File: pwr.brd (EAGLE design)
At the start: 50 x 58 mm, 40 parts, among them Q1 IPD65R600E6, T1 750811647, U1 UCC28700

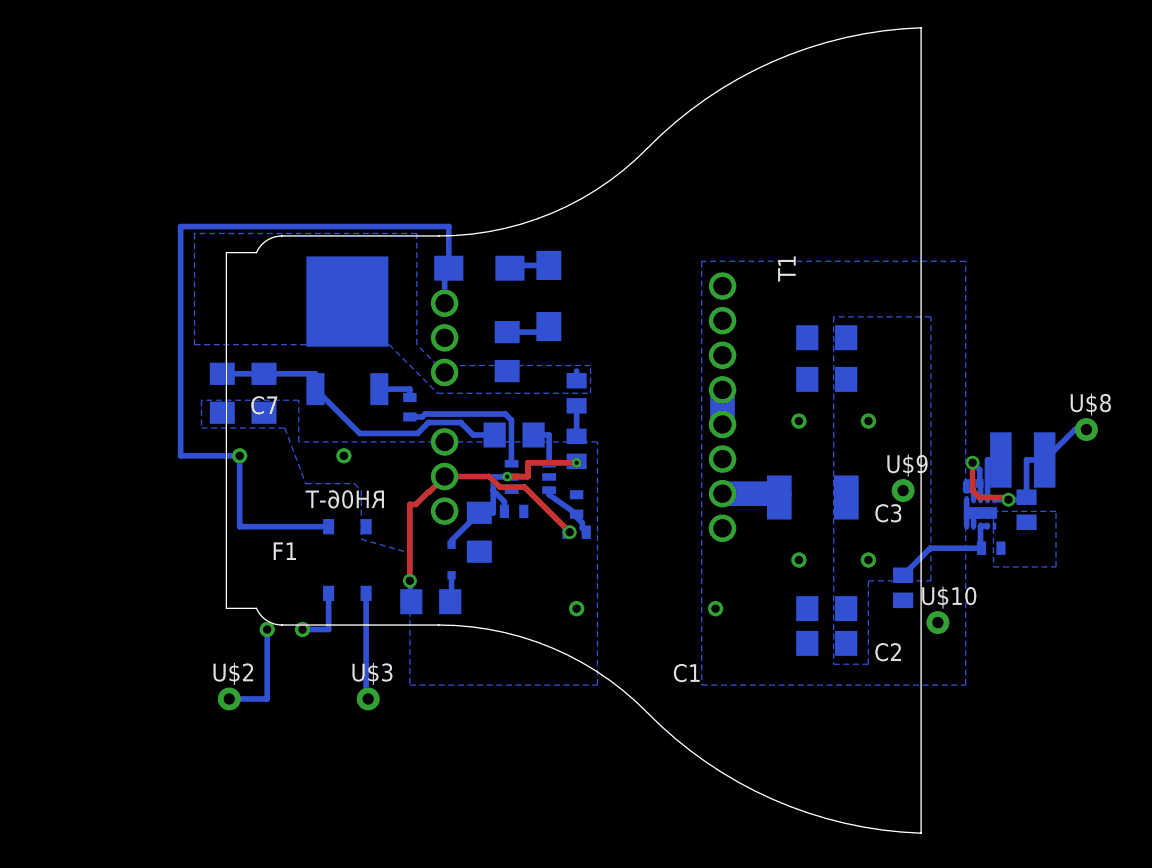
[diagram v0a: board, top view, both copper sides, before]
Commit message: getting close
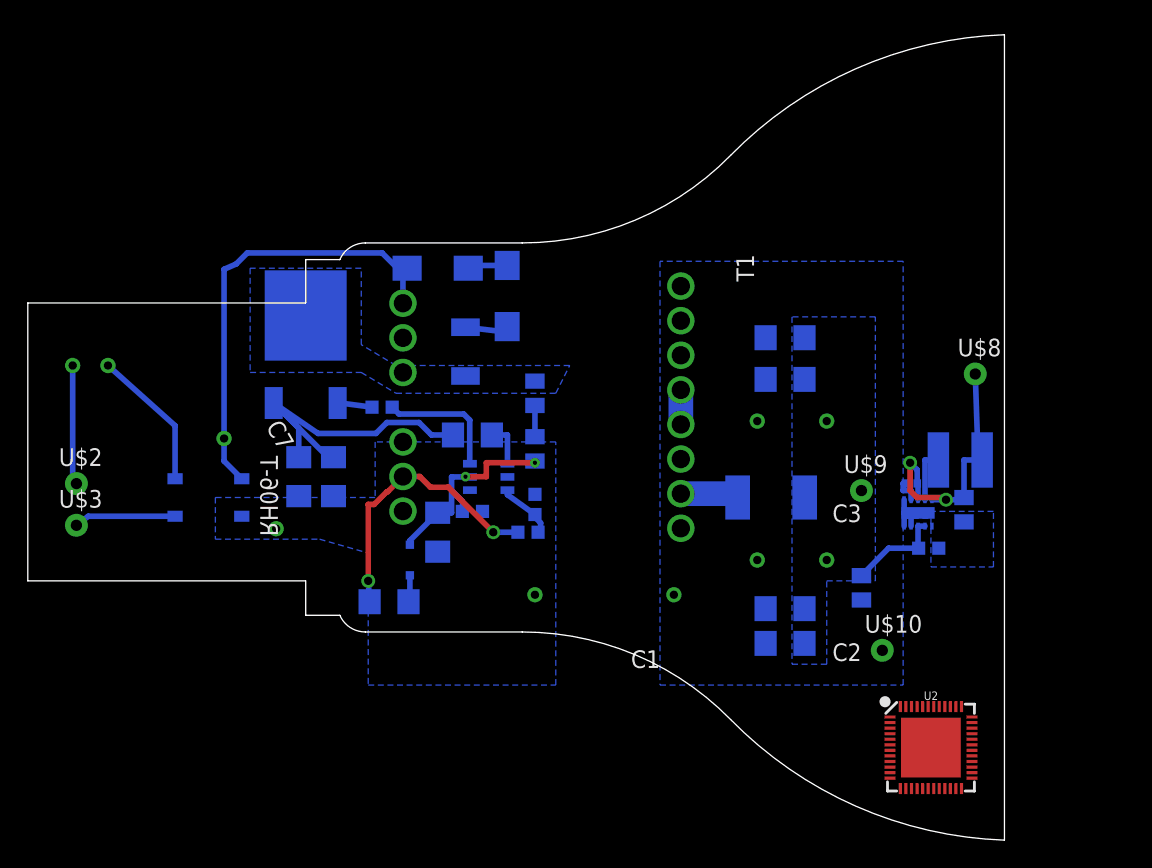
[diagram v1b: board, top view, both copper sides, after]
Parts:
- added U2: ESP3212, derek:QFN48-0.4MM
- C1: value DE1E3KX222MA4BL01 -> 2200pF
- C2, C3: value UHE1V221MPD6 -> 220µF
- C4, C5: value UMK316AB7475KL-T -> 4.7µF
- C6: value 08053C104KAT2A -> 0.1µF
- C7: value EEUED2G470 -> 47µF
- C8: value 06035C104KAT2A -> 0.1µF
- C9: value GRM31CR61H225KA88L -> 2.2µF
- C_1: value C1608X5R1V225K080AC -> 2.2µF
- C_2: value GRM21BR60J226ME39L -> 22µF
- Q1: value IPD65R600E6 -> IPD65R600C6
- R1, R101: value CRCW120610K0JNEA -> 10k
- R10, R9: value CSR1206FKR750 -> 0.75
- R11: value CRCW060319K6FKEA -> 19.6k
- R2: value CRCW120633R2FKEA -> 33.2; device derek:1206 -> derek:1210
- R3: value CRCW12064R70JNEA -> 4.7
- R4: value CRCW060375K0FKEA -> 75k
- R5, R6: value CRCW08053M30JNEA -> 3.3M
- R7: value CRCW06030000Z0EA -> 0.0
- R8: value CRCW1206698RFKEA -> 698
- R_1: value CRCW0402100KFKED -> 100k
- moved U$3 24.4 mm to (9.00, 38.5)
- moved F1 23.6 mm to (10.0, 50.0), flipped to the bottom, turned to 180 degrees
- moved U$2 19.0 mm to (9.00, 41.5)
- moved D3 11.0 mm to (18.5, 40.5), turned to 270 degrees
- moved U$8 8.94 mm to (73.7, 49.4)
- moved R10 8.14 mm to (25.0, 42.0)
- moved R9 7.81 mm to (27.5, 42.0)
- moved C_1 4.50 mm to (70.3, 36.9)
- moved C_2 4.50 mm to (72.9, 39.6)
- moved L_1 4.50 mm to (72.6, 43.2)
- moved R_1 4.50 mm to (69.1, 41.5)
- moved U_1 4.50 mm to (69.6, 39.4)
- moved U$10 4.47 mm to (67.0, 29.5)
- moved C7 3.61 mm to (21.5, 41.5), turned to 300 degrees
- moved R4 3.50 mm to (41.5, 38.0)
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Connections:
- net N$14: now also D5.C; no longer D5.1
- net N$16: now also D5.A; no longer D5.2
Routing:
- net N$3: track 57.4 -> 32.5 mm
- net N$1: track 4.48 -> 10.3 mm
- net 3.3V: track 18.1 -> 20.4 mm
- net N$15: track 22.7 -> 24.8 mm
- net N$13: track 10.7 -> 9.11 mm
- net 24V: track 8.61 -> 7.08 mm
- net N$17: track 21.2 -> 20.3 mm
- net N$11: track 7.73 -> 8.62 mm
- net GND: track 0.60 -> 0.00 mm
- net N$10: track 0.80 -> 0.26 mm
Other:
- board size 50 x 58 mm -> 70.3 x 58 mm
